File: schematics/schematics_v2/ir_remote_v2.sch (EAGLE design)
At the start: 25 parts, among them IC1 AP1117E50G, T11 TASTER3301, T12 TASTER3301, T13 TASTER3301, T14 TASTER3301, T15 TASTER3301

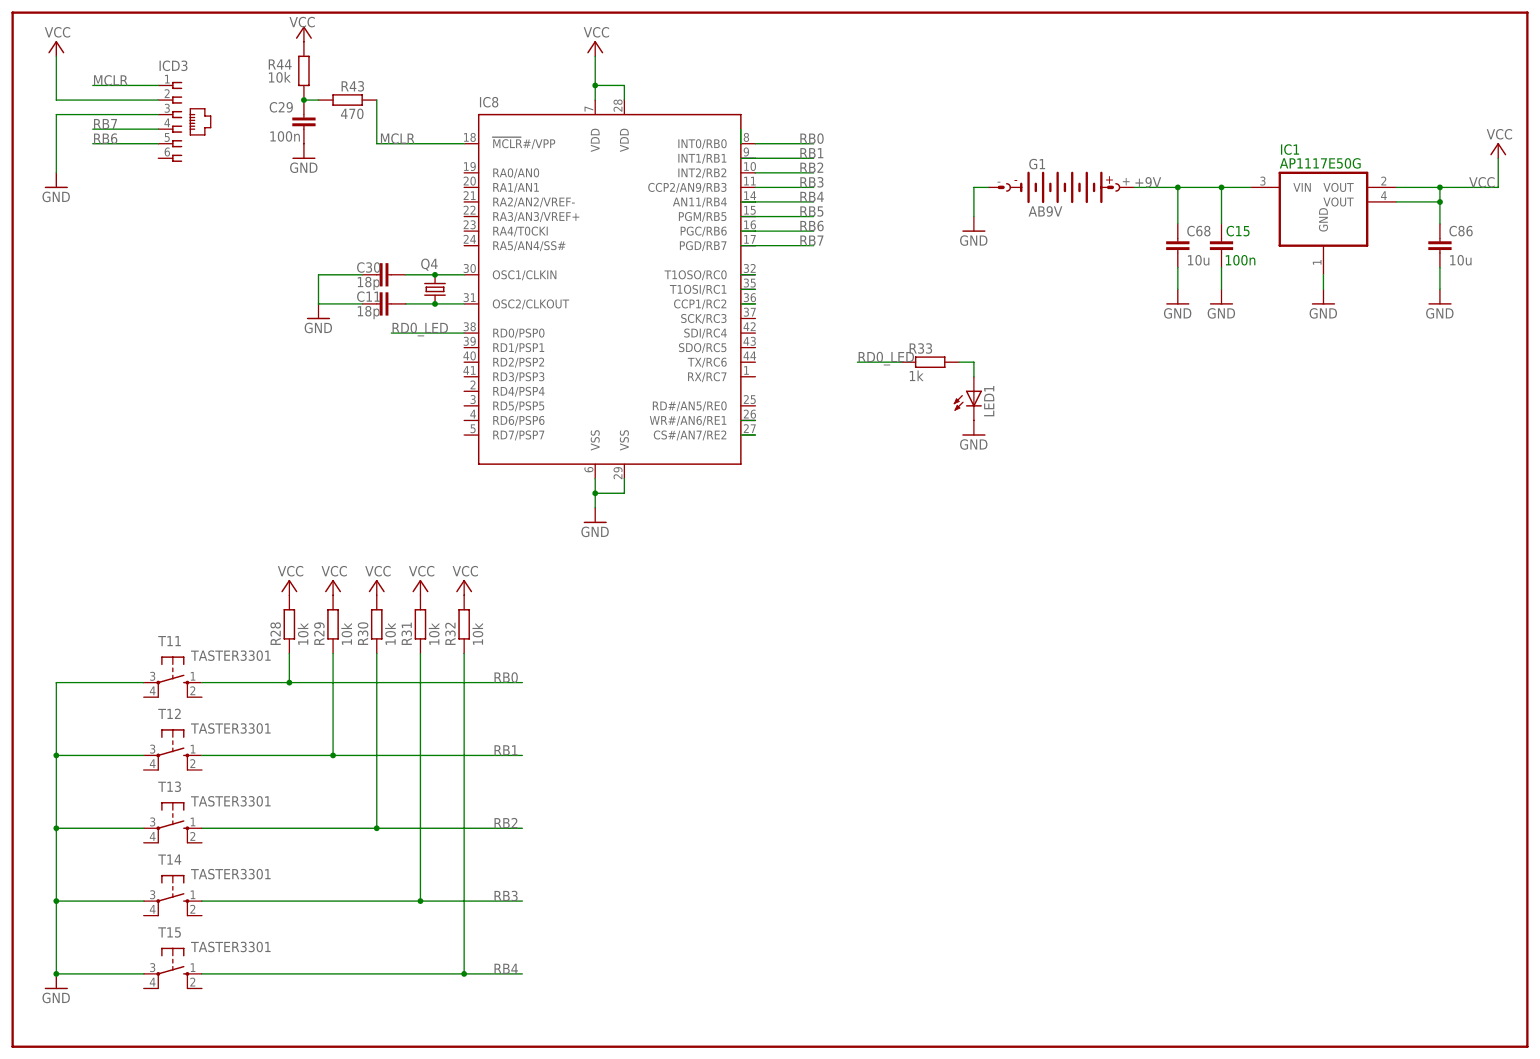
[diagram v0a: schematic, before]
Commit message: Clean up files in schematics v2
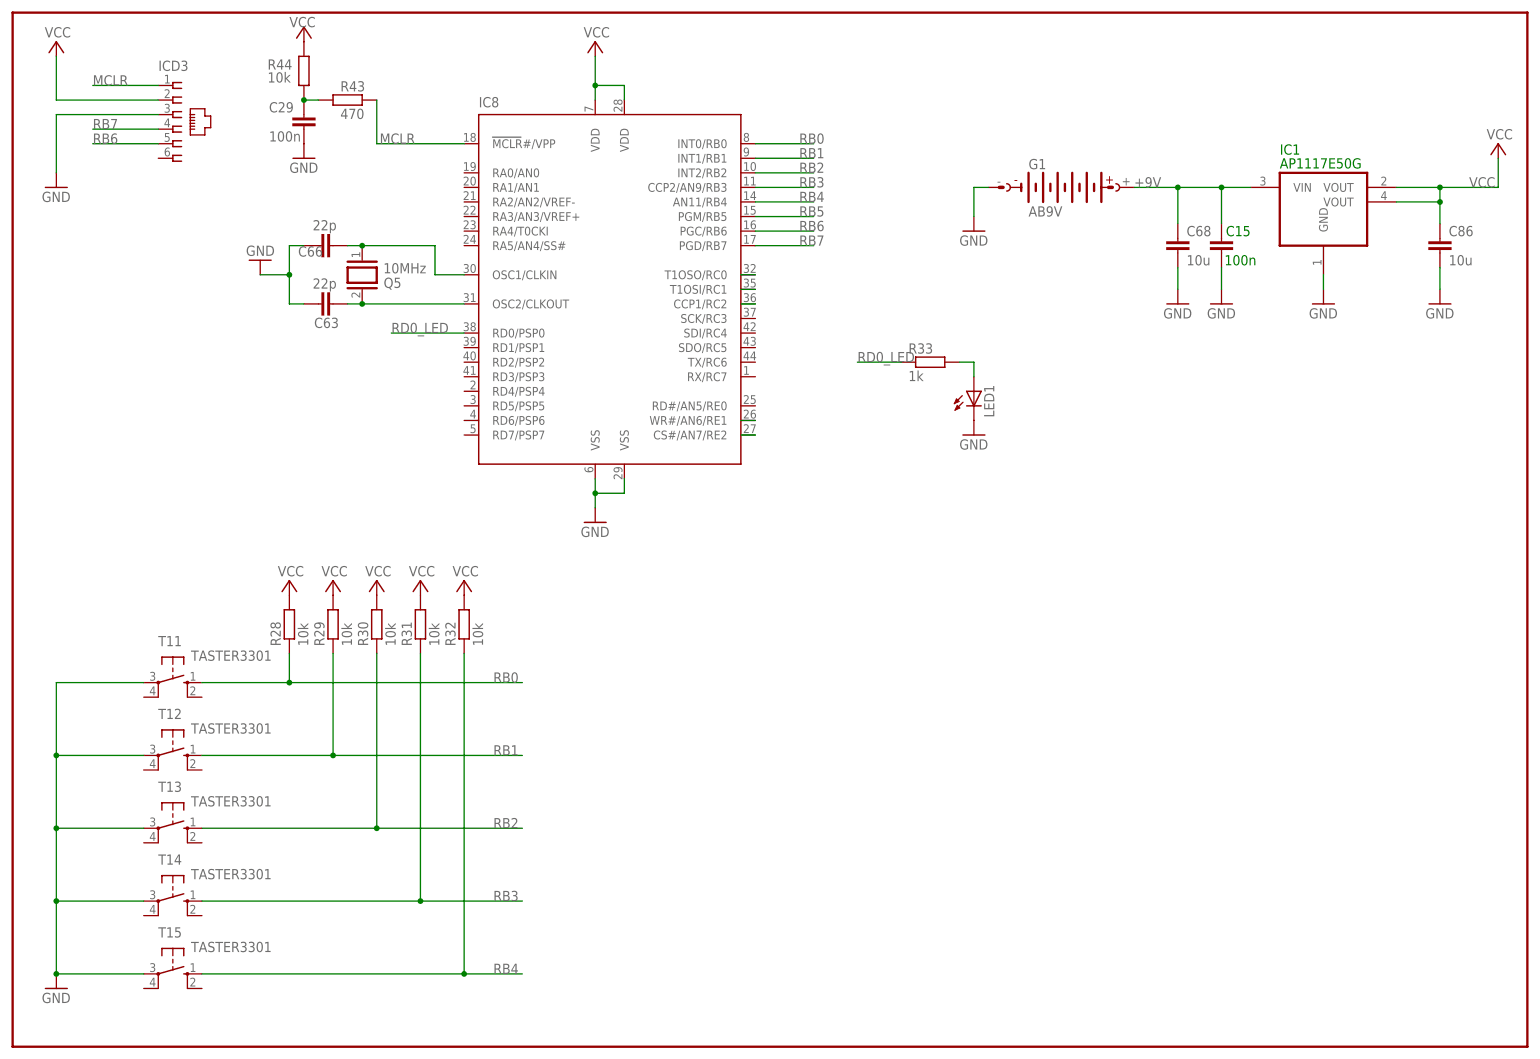
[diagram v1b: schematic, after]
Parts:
- removed C11, C30: 18p, rcl:C-EUC0805
- removed Q4: (no value), crystal:CRYTALHC49U-V
- added C63, C66: 22p, rcl:C-EUC0603_WE
- added Q5: 10MHz, Bernd:XTAL_HC5032
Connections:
- removed net N$25: C11.1, IC8.OSC2/CLKOUT, Q4.1
- removed net N$9: C30.1, IC8.OSC1/CLKIN, Q4.2
- new net N$47: C66.2, IC8.OSC1/CLKIN, Q5.1
- new net N$48: C63.2, IC8.OSC2/CLKOUT, Q5.2
- net GND: now also C63.1, C66.1; no longer C11.2, C30.2
